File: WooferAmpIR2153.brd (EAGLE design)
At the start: 142.2 x 47.3 mm, 70 parts

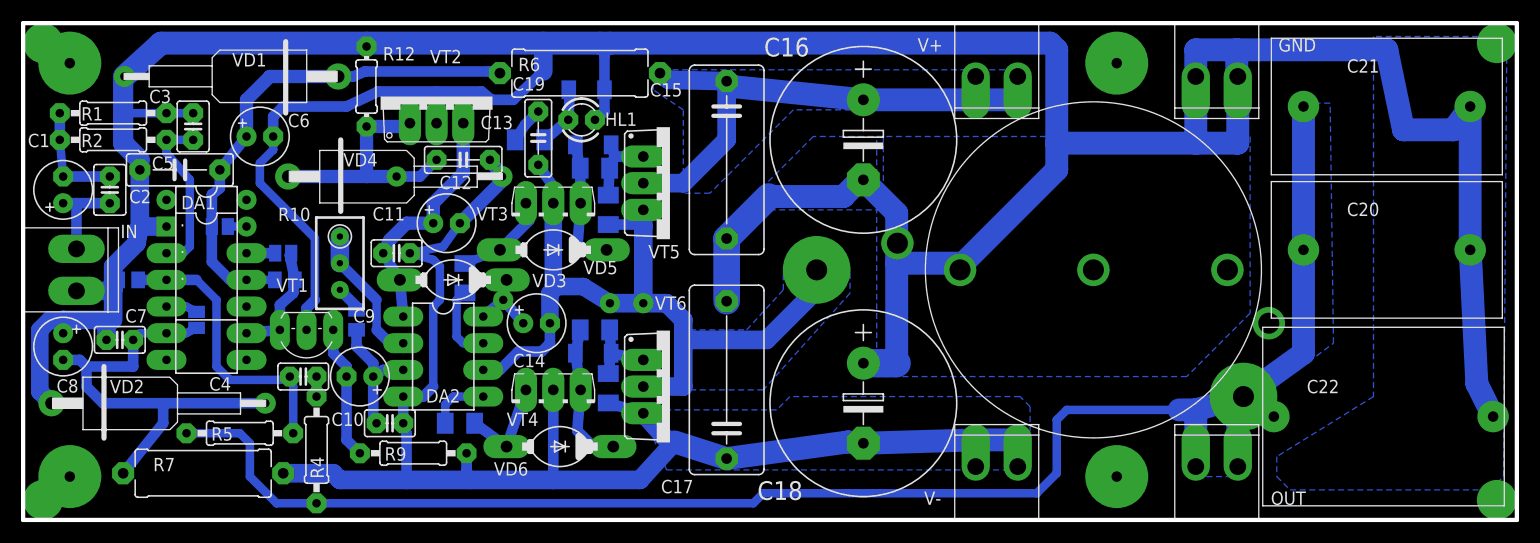
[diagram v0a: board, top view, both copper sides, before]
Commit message: 7
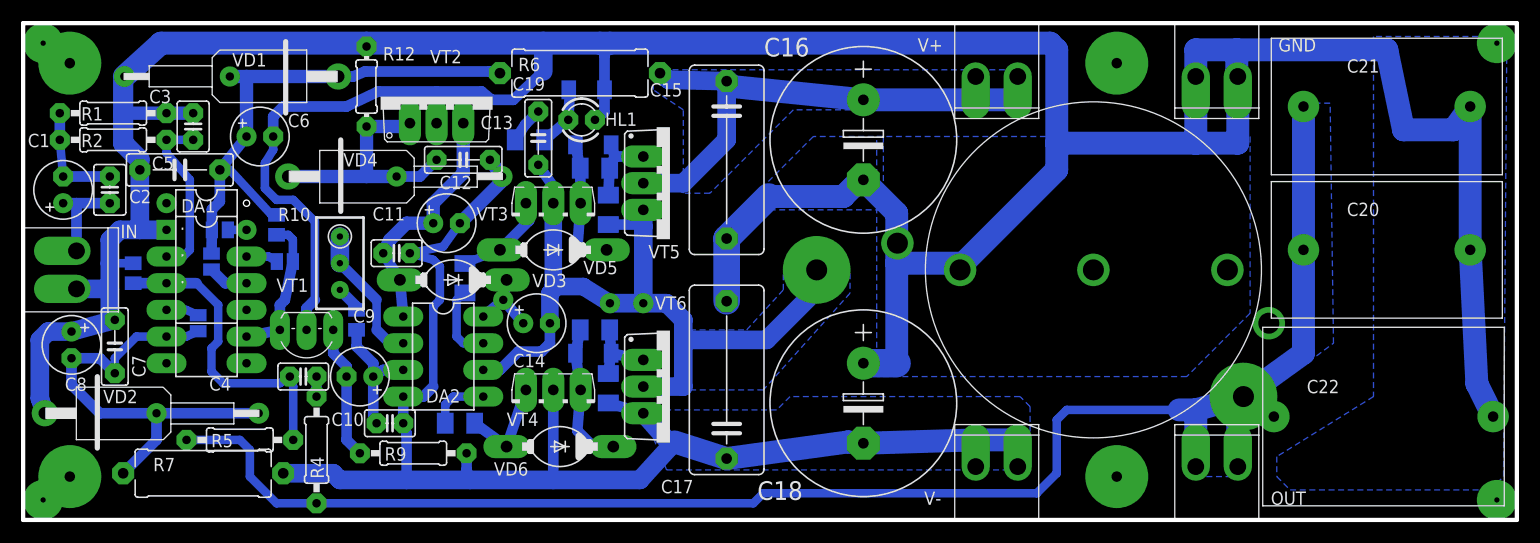
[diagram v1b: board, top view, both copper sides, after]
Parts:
- added SJ4: (no value), jumper:SJ
- C7: device resistor:C025-025X050 -> resistor:C050-025X075
- GND, OUT, V+, V-: value (none) -> CON_2PA
- IN: device DSS0:CON_PWR_2PIN4MM -> woofer:CON_PWRI_2PIN4MM
- moved R8 5.30 mm to (23.5, 26.5), turned to 90 degrees
- moved VD2 1.14 mm to (9.53, 8.57)
- moved C8 0.81 mm to (3.97, 15.1)
- moved SJ2 0.81 mm to (24.3, 23.0)
- moved C7 0.79 mm to (8.10, 14.9), turned to 90 degrees
- moved R3 0.79 mm to (9.84, 21.9), turned to 270 degrees
- moved R5 0.64 mm to (20.0, 6.03)
- moved SJ1 0.35 mm to (16.0, 17.1)
- moved DA1 0.32 mm to (16.8, 21.0)
- moved SJ3 0.32 mm to (18.1, 26.0)
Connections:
- new net N$8: DA1.11, SJ4.1
- net VC+: now also SJ4.2; no longer DA1.11
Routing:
- net N$8: track 0.00 -> 3.87 mm
- net CO: track 11.2 -> 13.9 mm
- net VC+: track 48.6 -> 51.2 mm, vias 0 -> 1
- net C-: track 27.6 -> 29.8 mm
- net L-OUT: track 158.7 -> 158.1 mm
- net VC-: track 43.5 -> 43.6 mm, vias 0 -> 1
